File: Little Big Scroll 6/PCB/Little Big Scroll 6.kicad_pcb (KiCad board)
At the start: 2 copper layers, 57.2 x 85 mm, 28 parts, among them J1 Conn_01x02, J2 Conn_01x02, SW1 SW_Push, SW2 SW_Push, SW3 SW_Push, SW4 SW_Push, SW5 SW_Push, SW6 SW_Push, SW7 Rotary_Encoder_Switch, U1 ProMicro

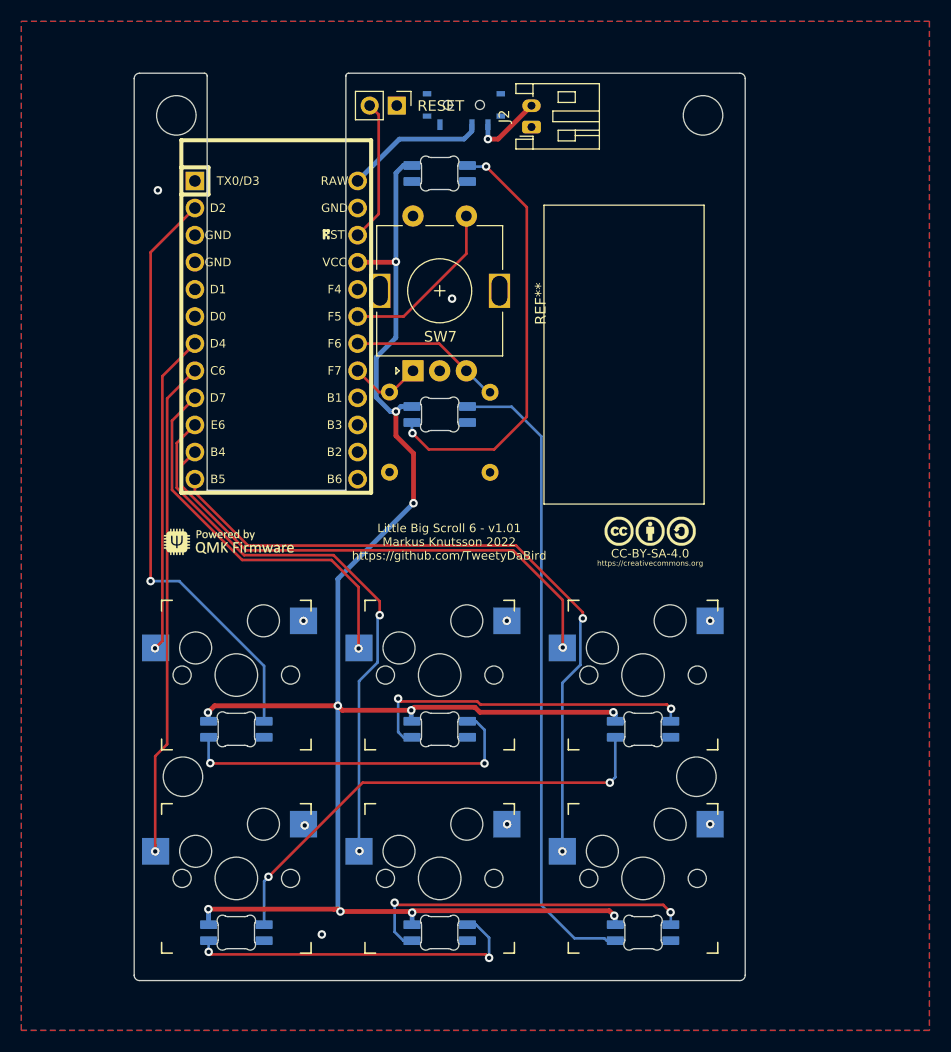
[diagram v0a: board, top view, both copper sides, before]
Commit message: LSB6 1.01
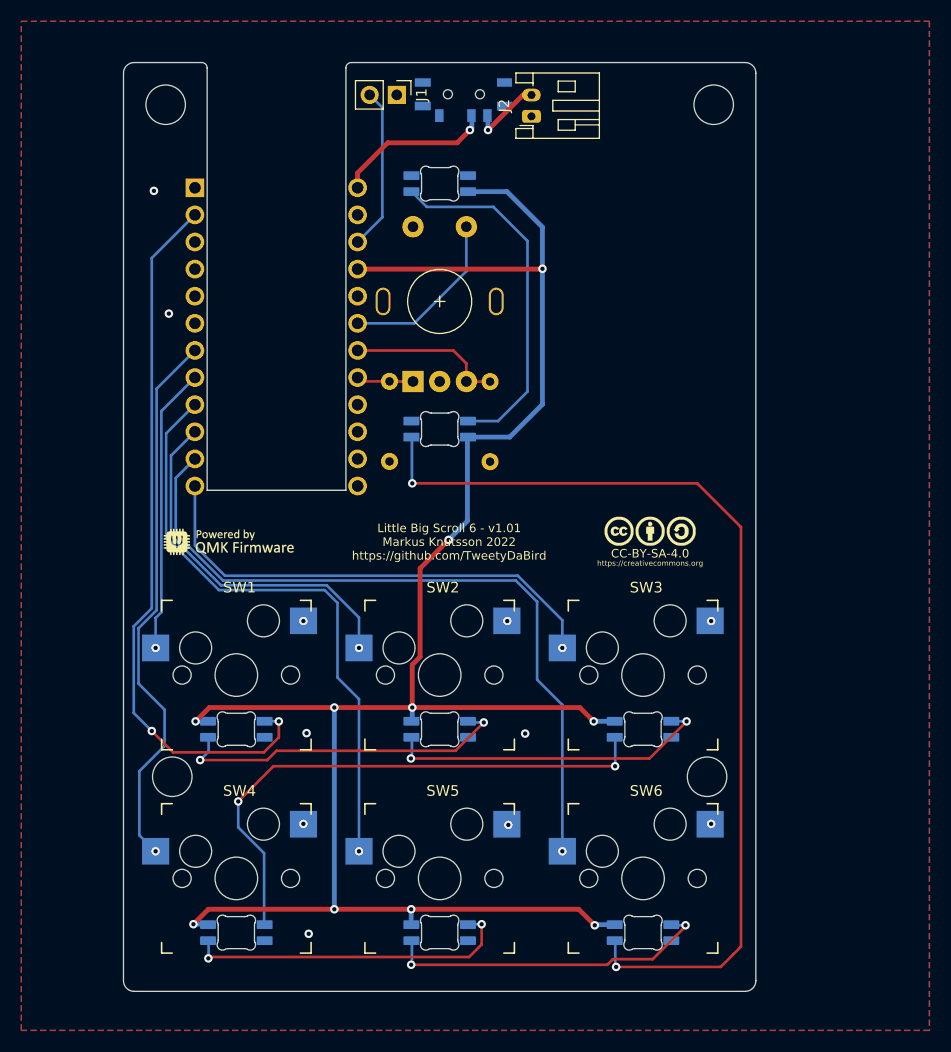
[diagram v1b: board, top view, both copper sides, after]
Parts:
- removed REF**: Lipo_battery_501528_1S_150mAh, Keyboard Library:Lipo_battery_501528_1S_150mAh
- C1, C2: value 100nF -> C_Small
- ENC1: renamed from SW7; value Rotary_Encoder_Switch -> Rotary_Encoder_Click; footprint Keyboard Library:RotaryEncoder_Alps_EC11E-Switch_Vertical_H20mm -> Keyboard Switches & Encoders:Encoder_Alps_EC11E_Small
- H1, H2, H3, H4: value Hole_PCB_M2-Spacer -> Spacer_PCB; footprint MountingHole:MountingHole_3.7mm -> Keyboard Switches & Encoders:Spacer PCB hole
- Logo1: renamed from Lic1; footprint CC_Licensing:CC_BY_SA_40 -> Logotypes:CC_BY_SA_40
- Logo2: renamed from Logo1; footprint QMK Logo:Powered_by_QMK -> Logotypes:Powered_by_QMK
- RGB1: renamed from LED1; footprint kicad-keyboard-parts:MX_SK6812MINI-E -> Keyboard Switches & Encoders:RGB_SK6812MINI-E
- RGB2: renamed from LED5; footprint kicad-keyboard-parts:MX_SK6812MINI-E -> Keyboard Switches & Encoders:RGB_SK6812MINI-E
- RGB3: renamed from LED2; footprint kicad-keyboard-parts:MX_SK6812MINI-E -> Keyboard Switches & Encoders:RGB_SK6812MINI-E
- RGB4: renamed from LED6; footprint kicad-keyboard-parts:MX_SK6812MINI-E -> Keyboard Switches & Encoders:RGB_SK6812MINI-E
- RGB5: renamed from LED3; footprint kicad-keyboard-parts:MX_SK6812MINI-E -> Keyboard Switches & Encoders:RGB_SK6812MINI-E
- RGB6: renamed from LED7; footprint kicad-keyboard-parts:MX_SK6812MINI-E -> Keyboard Switches & Encoders:RGB_SK6812MINI-E
- RGB7: renamed from LED4; footprint kicad-keyboard-parts:MX_SK6812MINI-E -> Keyboard Switches & Encoders:RGB_SK6812MINI-E
- RGB8: renamed from LED8; footprint kicad-keyboard-parts:MX_SK6812MINI-E -> Keyboard Switches & Encoders:RGB_SK6812MINI-E
- S1: footprint Keyboard Library:MSK12C02 -> Keyboard Switches & Encoders:MSK12C02
- SW1, SW2, SW3, SW4, SW5, SW6: value SW_Push -> SW_MX_HS; footprint keyswitches:Kailh_socket_MX_RGB -> Keyboard Switches & Encoders:SW_MX_HotSwap
- U1: footprint Keebio-Parts:ArduinoProMicro -> Keyboard Library:ArduinoProMicro-BackSide
- moved RGB6 11.5 mm to (110.3, 85.2), turned to 180 degrees
- moved RGB8 11.1 mm to (110.3, 62.2), turned to 180 degrees
- moved H3 1.41 mm to (135.9, 49.7)
- moved H4 1.41 mm to (84.6, 49.7)
- moved C1 1.00 mm to (105.6, 75.7)
- moved C2 1.00 mm to (115.0, 83.2)
- moved ENC1 1.00 mm to (110.3, 68.2)
- moved H1 1.00 mm to (85.2, 112.7)
- moved H2 1.00 mm to (135.3, 112.7)
- moved J1 1.00 mm to (106.2, 48.8)
- moved J2 1.00 mm to (118.9, 50.8)
- moved S1 1.00 mm to (112.5, 48.8)
- moved U1 0.64 mm to (95.0, 71.5)
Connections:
- SW1 pad 1: GND -> Key1
- SW1 pad 2: Key1 -> GND
- SW2 pad 1: GND -> Key2
- SW2 pad 2: Key2 -> GND
- SW3 pad 1: GND -> Key3
- SW3 pad 2: Key3 -> GND
- SW4 pad 1: GND -> Key4
- SW4 pad 2: Key4 -> GND
- SW5 pad 1: GND -> Key5
- SW5 pad 2: Key5 -> GND
- SW6 pad 1: GND -> Key6
- SW6 pad 2: Key6 -> GND
- U1 pad 10: Key5 -> Key2
- U1 pad 11: Key3 -> Key6
- U1 pad 12: Key6 -> Key3
- U1 pad 7: Key1 -> Key4
- U1 pad 8: Key4 -> Key1
- U1 pad 9: Key2 -> Key5
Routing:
- net Net-(RGB4-Pad2): track 60.3 -> 91.1 mm, vias 0 -> 2
- net VCC: track 165.3 -> 183.5 mm, vias 11 -> 10
- net RGB: track 55.8 -> 67.6 mm, vias 1 -> 2
- net Net-(RGB5-Pad2): track 44.7 -> 51.9 mm
- net Net-(RGB6-Pad2): track 40.4 -> 33.6 mm, vias 2 -> 0
- net Key4: track 46.6 -> 51.7 mm
- net Key1: track 30.1 -> 26.9 mm
- net Key6: track 65.4 -> 68.6 mm, vias 2 -> 1
- net Key3: track 48.3 -> 45.5 mm
- net Key2: track 36.5 -> 34.3 mm
- net Key5: track 54.2 -> 56.2 mm, vias 2 -> 1
- net Net-(U1-Pad22): track 13.3 -> 15.2 mm
- net BAT+: track 13.3 -> 15.2 mm, vias 0 -> 1
- net EncA: track 6.84 -> 5.34 mm
- net Net-(RGB1-Pad2): track 33.3 -> 32.1 mm
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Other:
- board size 57.2 x 85 mm -> 59.2 x 87 mm
- board text added: "Mount ProMicro on bottom of PCB, components facing up."
- board text removed: "For best results, mount ProMicro on bottom of PCB, components facing up."
